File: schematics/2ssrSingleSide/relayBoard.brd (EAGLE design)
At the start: 100 x 80 mm, 24 parts, among them K1 AQG12105, K2 AQG12105

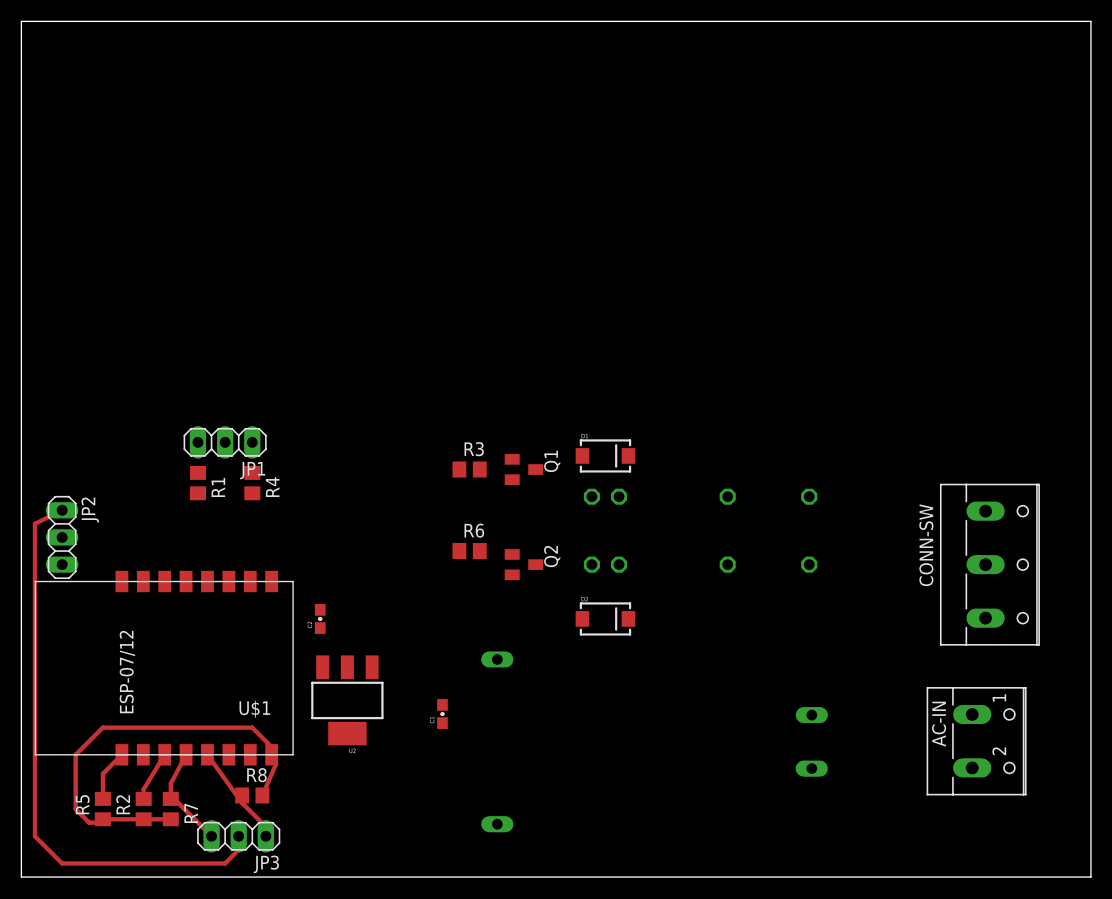
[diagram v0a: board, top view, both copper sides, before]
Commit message: moved schematics and board
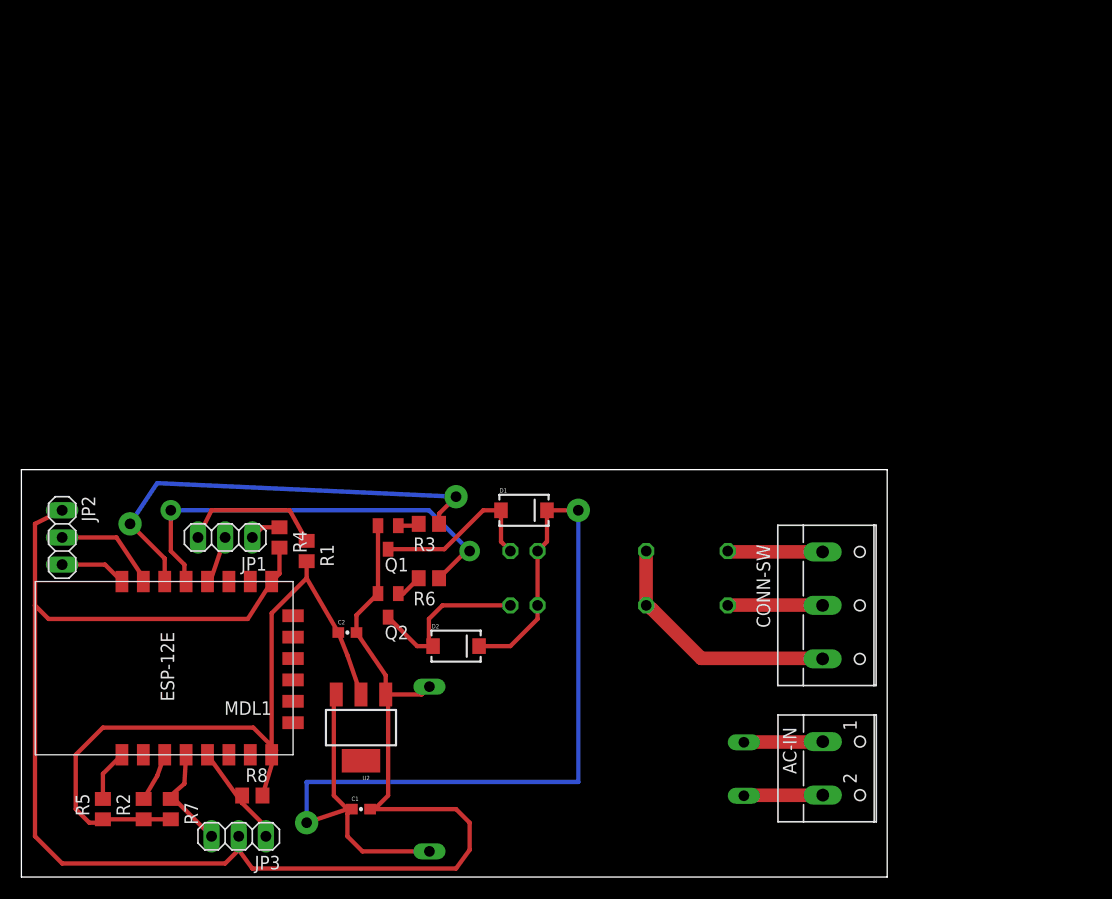
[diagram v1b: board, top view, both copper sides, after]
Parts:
- removed U$1: ESP8266_ESP-12, ESP8266-ESP12:ESP8266-ESP12
- added MDL1: (no value), ESP8266-ESP12E:ESP8266-ESP12E
- moved CONN-SW 15.7 mm to (76.2, 25.4)
- moved Q1 14.2 mm to (34.3, 31.8), turned to 180 degrees
- moved AC-IN 14.2 mm to (76.2, 10.2)
- moved D2 14.2 mm to (40.6, 21.6)
- moved Q2 13.3 mm to (34.3, 25.4), turned to 180 degrees
- moved R1 12.0 mm to (26.7, 30.5)
- moved C1 11.7 mm to (31.8, 6.35), turned to 0 degrees
- moved K1 9.16 mm to (55.9, 30.5)
- moved D1 9.16 mm to (47.0, 34.3)
- moved JP1 8.89 mm to (19.1, 31.8)
- moved K2 8.52 mm to (55.9, 25.4)
- moved U$4 6.84 mm to (69.8, 0.00)
- moved R3 6.35 mm to (38.1, 33.0), turned to 180 degrees
- moved R4 5.68 mm to (24.1, 31.8)
- moved R6 4.58 mm to (38.1, 27.9), turned to 180 degrees
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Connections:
- removed net AC-SW-L: CONN-SW.1, K1.O1, K2.O1
- removed net CH_PD: R2.2, U$1.11
- removed net GPIO2: U$1.3
- removed net LOAD1: CONN-SW.2, K1.O2
- removed net LOAD2: CONN-SW.3, K2.O2
- removed net N$4: R5.2, U$1.9
- new net LOAD1L: CONN-SW.1, K1.O2
- new net LOAD2L: CONN-SW.2, K2.O2
- new net LOADN: CONN-SW.3, K1.O1, K2.O1
- new net N$6: MDL1.1, R5.2
- new net N$9: MDL1.3, R2.2
- net 3V3: now also MDL1.8; no longer D1.C, D2.C, K1.+, K2.+, U$1.16
- net 5V: now also D1.C, D2.C, K1.+, K2.+
- net GND: now also MDL1.9; no longer U$1.1
- net GPIO0: now also MDL1.12; no longer U$1.4
- net GPIO14: now also MDL1.5; no longer U$1.13
- net GPIO16: now also MDL1.4; no longer U$1.12
- net GPIO4: now also MDL1.13, R6.1; no longer R3.1, U$1.6
- net GPIO5: now also MDL1.14, R3.1; no longer R6.1, U$1.5
- net RXD: now also MDL1.15; no longer U$1.7
- net TXD: now also MDL1.16; no longer U$1.8
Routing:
- net 5V: track 0.00 -> 101.3 mm, vias 0 -> 2
- net GND: track 53.9 -> 150.9 mm
- net GPIO5: track 0.00 -> 42.5 mm, vias 0 -> 2
- net GPIO4: track 0.00 -> 40.7 mm, vias 0 -> 2
- net 3V3: track 39.6 -> 71.2 mm
- net LOADN: track 0.00 -> 23.6 mm
- net N$10: track 0.00 -> 16.2 mm
- net N$7: track 0.00 -> 16.2 mm
- net N$1: track 0.00 -> 13.4 mm
- net RXD: track 0.00 -> 9.98 mm
- net LOAD1L: track 0.00 -> 8.93 mm
- net LOAD2L: track 0.00 -> 8.89 mm
- net N$5: track 0.00 -> 7.41 mm
- net N$2: track 0.00 -> 7.40 mm
- net TXD: track 0.00 -> 6.24 mm
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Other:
- board size 100 x 80 mm -> 81 x 38.1 mm
